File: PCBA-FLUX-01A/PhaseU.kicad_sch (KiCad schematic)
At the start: 60 parts, among them Q2 IPT015N10N5, Q3 IPT015N10N5, Q4 IPT015N10N5, Q5 IPT015N10N5, Q6 BC817, U2 INA240A2DR, U3 UCC27211AQDDARQ1, U4 TLV9001

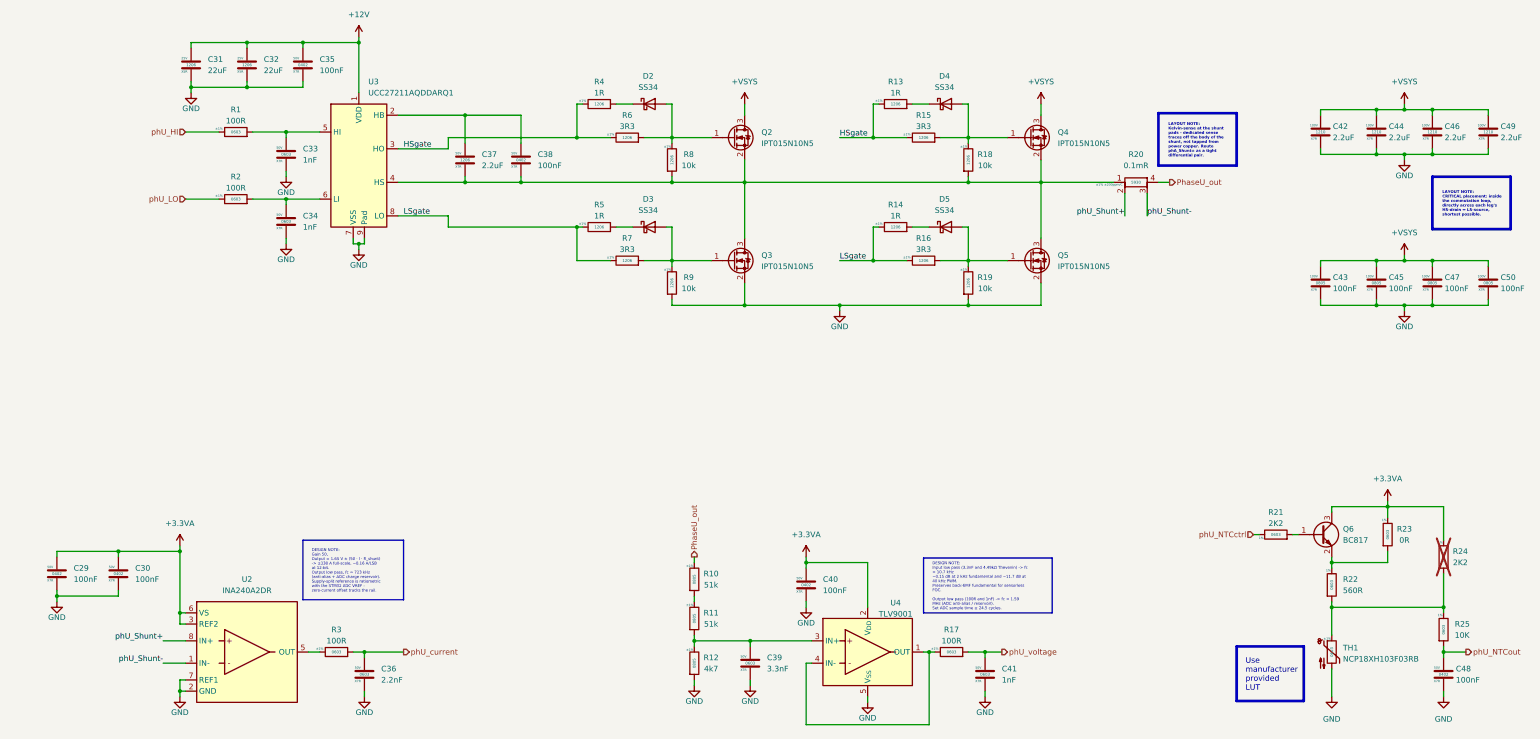
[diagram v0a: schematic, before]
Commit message: Changes were made
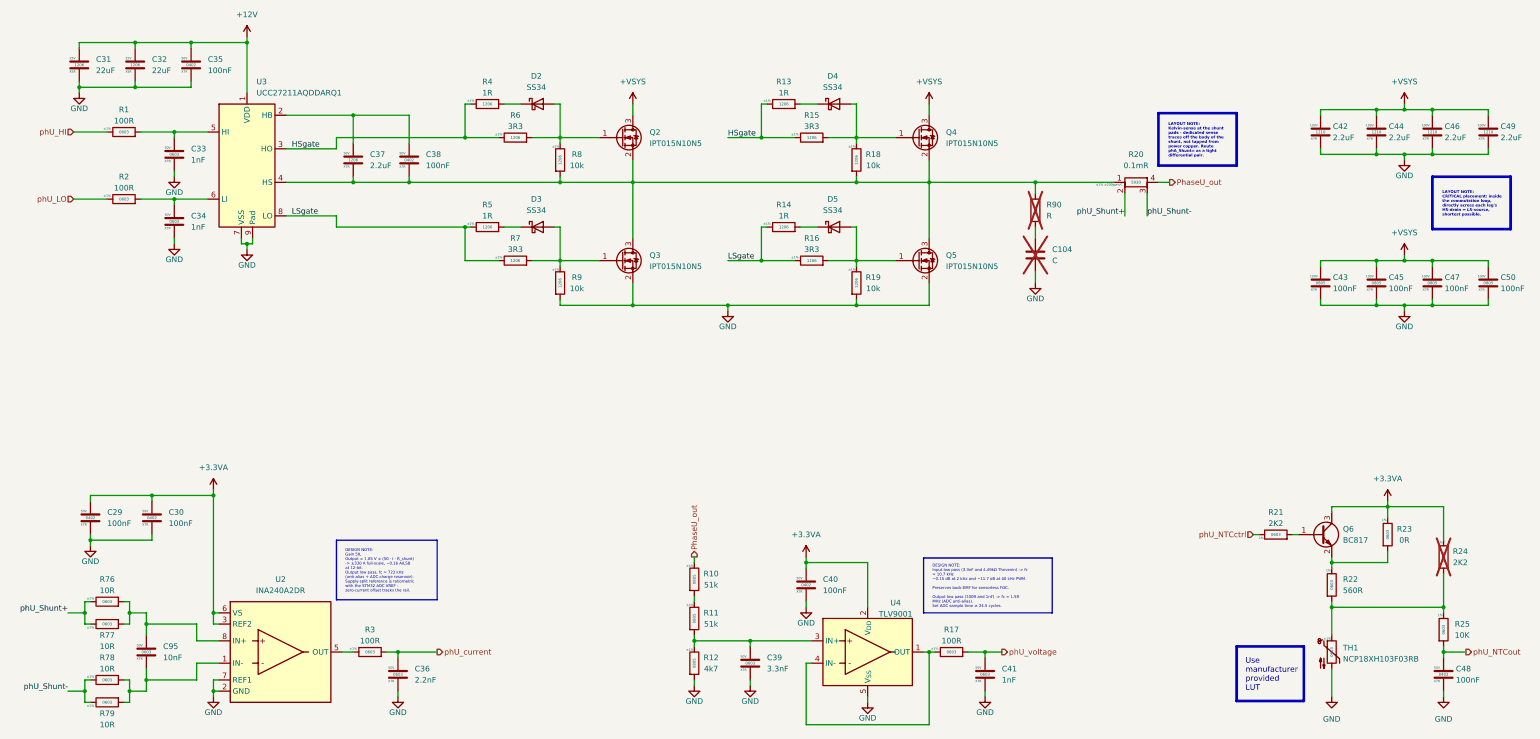
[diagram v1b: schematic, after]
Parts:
- added C104: C, Capacitor_THT:C_Rect_L9.0mm_W6.4mm_P7.50mm_MKT, symbol Device:C
- added C95: 10nF, Capacitor_SMD:C_0603_1608Metric, symbol Device:C
- added R76, R77, R78, R79: 10R, Resistor_SMD:R_0805_2012Metric, symbol Device:R
- added R90: R, Resistor_SMD:R_1218_3246Metric, symbol Device:R
- R1, R17, R2: footprint Resistor_SMD:R_0805_2012Metric -> Resistor_SMD:R_0603_1608Metric
- R3: footprint Resistor_SMD:R_0805_2012Metric -> palmkiLib:R_0603_1608Metric
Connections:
- net GND: now also C104.2
- net phU_Shunt+: now also R76.1, R77.1; no longer U2.8 (IN+)
- net phU_Shunt-: now also R78.1, R79.1; no longer U2.1 (IN-)
- net at C37.2, C38.2, Q2.2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: now also R90.1
- new net: C95.1, R76.2, R77.2, U2.8 (IN+)
- new net: C95.2, R78.2, R79.2, U2.1 (IN-)
- new net: C104.1, R90.2
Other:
- moved on the sheet: C29, C30, C31, C32, C33, C34, C35, C36, C37, C38, D2, D3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
